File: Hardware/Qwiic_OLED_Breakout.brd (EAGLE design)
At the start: 27.3 x 34.3 mm, 29 parts

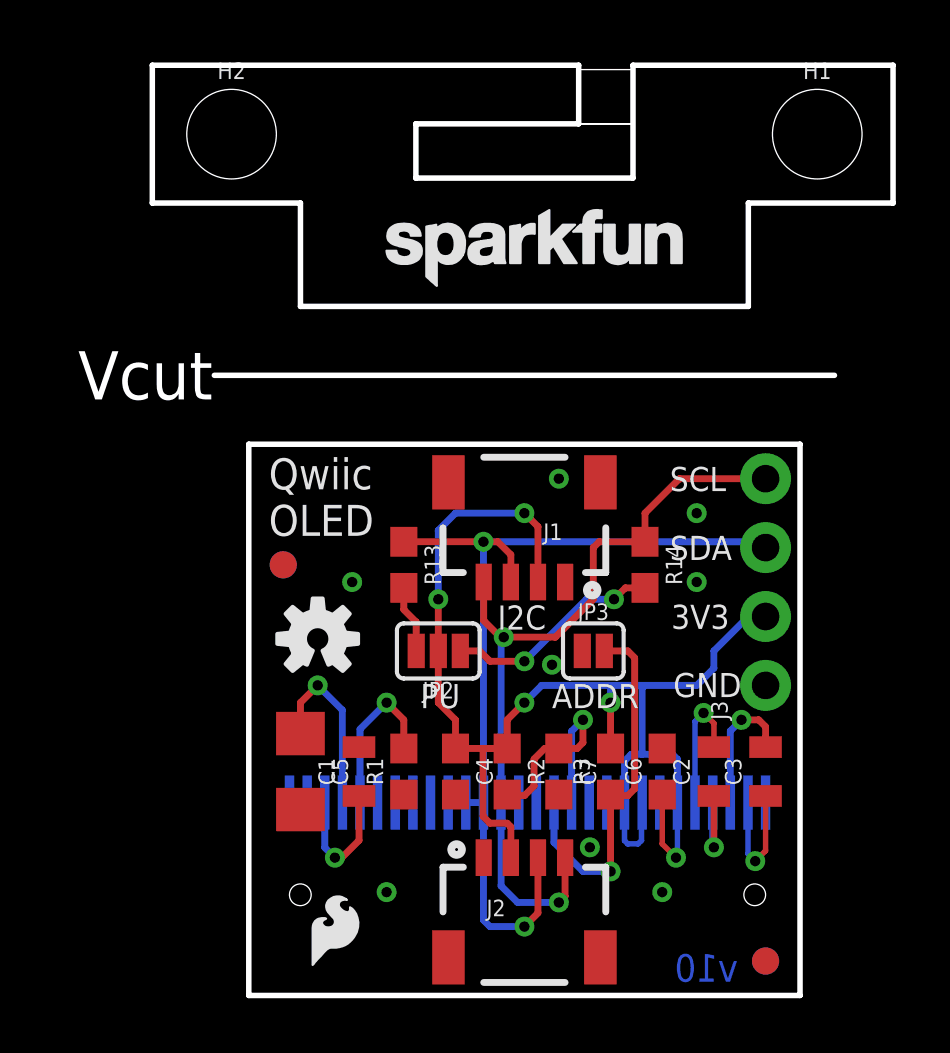
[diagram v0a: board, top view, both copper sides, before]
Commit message: fixed vscore
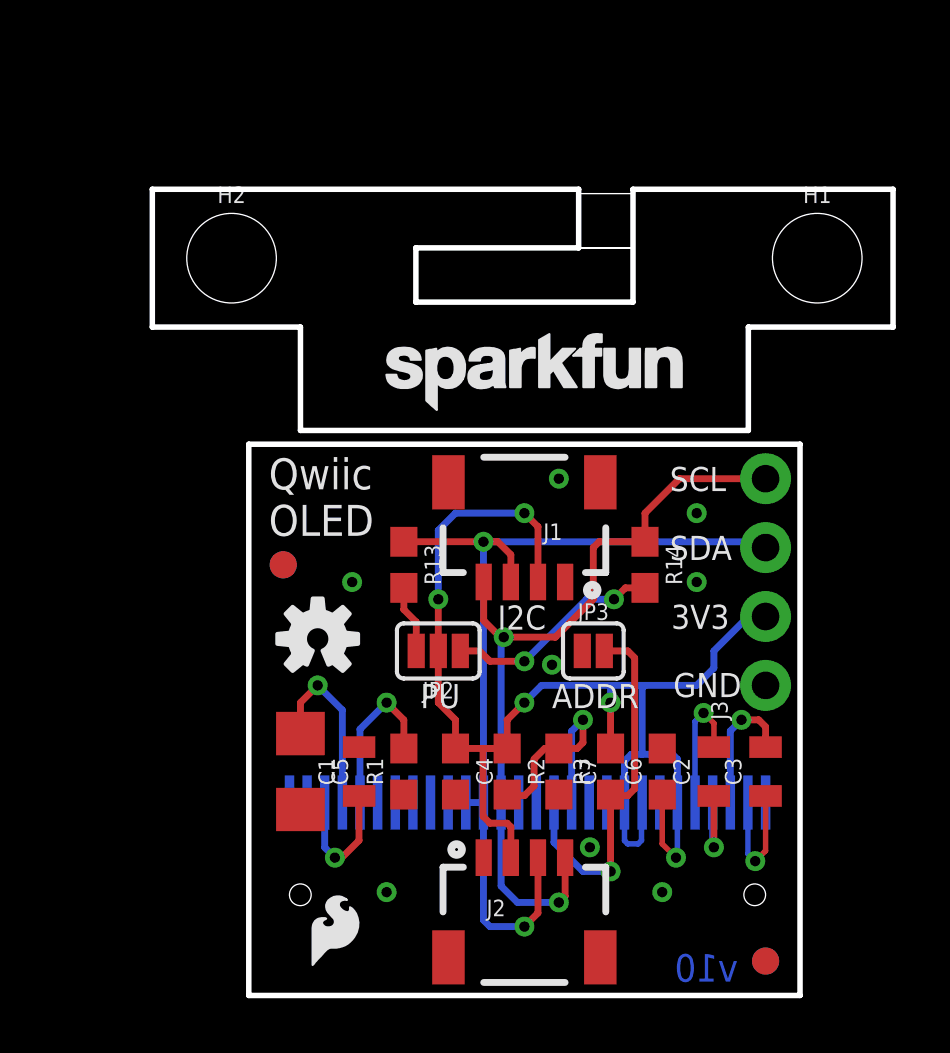
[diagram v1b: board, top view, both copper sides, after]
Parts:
- moved H1 4.57 mm to (21.0, 27.2)
- moved H2 4.57 mm to (-0.64, 27.2)
- moved LOGO4 4.57 mm to (4.57, 21.1)
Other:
- board size 27.3 x 34.3 mm -> 27.3 x 29.7 mm
- board text removed: "Vcut"
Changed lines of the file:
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@@
 <setting verticaltext="up"/>
 </settings>
-<grid distance="0.05" unitdist="inch" unit="inch" style="lines" multiple="1" display="yes" altdistance="0.005" altunitdist="inch" altunit="inch"/>
+<grid distance="0.01" unitdist="inch" unit="inch" style="lines" multiple="1" display="yes" altdistance="0.005" altunitdist="inch" altunit="inch"/>
 <layers>
 <layer number="1" name="Top" color="4" fill="1" visible="yes" active="yes"/>
@@
 <wire x1="0" y1="20.32" x2="0" y2="0" width="0.2032" layer="20"/>
 <wire x1="0" y1="0" x2="20.32" y2="0" width="0.2032" layer="20"/>
-<wire x1="-3.556" y1="34.29" x2="-3.556" y2="29.21" width="0.2032" layer="20"/>
-<wire x1="-3.556" y1="29.21" x2="1.905" y2="29.21" width="0.2032" layer="20"/>
-<wire x1="18.415" y1="29.21" x2="23.749" y2="29.21" width="0.2032" layer="20"/>
-<wire x1="23.749" y1="29.21" x2="23.749" y2="34.29" width="0.2032" layer="20"/>
-<rectangle x1="6.16" y1="30.13" x2="14.16" y2="32.13" layer="46" rot="R180"/>
-<rectangle x1="12.16" y1="32.13" x2="14.16" y2="34.13" layer="46" rot="R180"/>
-<wire x1="12.16" y1="34.29" x2="12.16" y2="32.13" width="0.2032" layer="20"/>
-<wire x1="12.16" y1="32.13" x2="6.16" y2="32.13" width="0.2032" layer="20"/>
-<wire x1="6.16" y1="32.13" x2="6.16" y2="30.13" width="0.2032" layer="20"/>
-<wire x1="6.16" y1="30.13" x2="14.16" y2="30.13" width="0.2032" layer="20"/>
-<wire x1="12.16" y1="34.29" x2="-3.556" y2="34.29" width="0.2032" layer="20"/>
-<wire x1="14.163040625" y1="30.134559375" x2="14.163040625" y2="34.29" width="0.2032" layer="20"/>
-<wire x1="14.163040625" y1="34.29" x2="23.749" y2="34.29" width="0.2032" layer="20"/>
+<wire x1="-3.556" y1="29.718" x2="-3.556" y2="24.638" width="0.2032" layer="20"/>
+<wire x1="-3.556" y1="24.638" x2="1.905" y2="24.638" width="0.2032" layer="20"/>
+<wire x1="18.415" y1="24.638" x2="23.749" y2="24.638" width="0.2032" layer="20"/>
+<wire x1="23.749" y1="24.638" x2="23.749" y2="29.718" width="0.2032" layer="20"/>
+<rectangle x1="6.16" y1="25.558" x2="14.16" y2="27.558" layer="46" rot="R180"/>
+<rectangle x1="12.16" y1="27.558" x2="14.16" y2="29.558" layer="46" rot="R180"/>
+<wire x1="12.16" y1="29.718" x2="12.16" y2="27.558" width="0.2032" layer="20"/>
+<wire x1="12.16" y1="27.558" x2="6.16" y2="27.558" width="0.2032" layer="20"/>
+<wire x1="6.16" y1="27.558" x2="6.16" y2="25.558" width="0.2032" layer="20"/>
+<wire x1="6.16" y1="25.558" x2="14.16" y2="25.558" width="0.2032" layer="20"/>
+<wire x1="12.16" y1="29.718" x2="-3.556" y2="29.718" width="0.2032" layer="20"/>
+<wire x1="14.163040625" y1="25.562559375" x2="14.163040625" y2="29.718" width="0.2032" layer="20"/>
+<wire x1="14.163040625" y1="29.718" x2="23.749" y2="29.718" width="0.2032" layer="20"/>
 <text x="8.89" y="-27.94" size="1.778" layer="51" font="vector">Joel Bartlett</text>
-<dimension x1="-3.81" y1="34.29" x2="-3.81" y2="0" x3="-15.24" y3="17.145" textsize="1.778" layer="47" unit="inch"/>
-<dimension x1="-3.556" y1="34.29" x2="23.749" y2="34.29" x3="10.0965" y3="40.64" textsize="1.778" layer="47" unit="inch"/>
-<dimension x1="-0.635" y1="31.75" x2="20.955" y2="31.75" x3="10.16" y3="36.83" textsize="1.778" layer="47" unit="inch"/>
-<dimension x1="0" y1="0" x2="0" y2="31.75" x3="-11.43" y3="15.875" textsize="1.778" layer="47" unit="inch"/>
+<dimension x1="-3.81" y1="29.718" x2="-3.81" y2="0" x3="-15.24" y3="14.859" textsize="1.778" layer="47" unit="inch"/>
+<dimension x1="-3.556" y1="29.718" x2="23.749" y2="29.718" x3="10.0965" y3="36.068" textsize="1.778" layer="47" unit="inch"/>
+<dimension x1="-0.635" y1="27.178" x2="20.955" y2="27.178" x3="10.16" y3="32.258" textsize="1.778" layer="47" unit="inch"/>
+<dimension x1="0" y1="0" x2="0" y2="27.178" x3="-11.43" y3="13.589" textsize="1.778" layer="47" unit="inch"/>
 <text x="12.7" y="-30.48" size="1.778" layer="51" font="vector">Andy England</text>
-<wire x1="-1.27" y1="22.86" x2="21.59" y2="22.86" width="0.2032" layer="20"/>
-<wire x1="1.905" y1="29.21" x2="1.905" y2="25.4" width="0.2032" layer="20"/>
-<wire x1="1.905" y1="25.4" x2="18.415" y2="25.4" width="0.2032" layer="20"/>
-<wire x1="18.415" y1="25.4" x2="18.415" y2="29.21" width="0.2032" layer="20"/>
+<wire x1="1.905" y1="24.638" x2="1.905" y2="20.828" width="0.2032" layer="20"/>
+<wire x1="1.905" y1="20.828" x2="18.415" y2="20.828" width="0.2032" layer="20"/>
+<wire x1="18.415" y1="20.828" x2="18.415" y2="24.638" width="0.2032" layer="20"/>
 <wire x1="0" y1="20.32" x2="20.32" y2="20.32" width="0.2032" layer="20"/>
-<text x="-3.81" y="22.86" size="1.778" layer="20" align="center">Vcut</text>
-<dimension x1="-6.35" y1="22.86" x2="-6.35" y2="0" x3="-7.62" y3="11.43" textsize="1.778" layer="20" unit="inch"/>
 </plain>
 <attributes>
@@
 </element>
 <element name="JP2" library="SparkFun-Jumpers" package="SMT-JUMPER_3_2-NC_PASTE_SILK" value="" x="6.985" y="12.7" rot="R180"/>
-<element name="H1" library="SparkFun-Hardware" package="STAND-OFF" value="STAND-OFF" x="20.955" y="31.75"/>
-<element name="H2" library="SparkFun-Hardware" package="STAND-OFF" value="STAND-OFF" x="-0.635" y="31.75"/>
+<element name="H1" library="SparkFun-Hardware" package="STAND-OFF" value="STAND-OFF" x="20.955" y="27.178"/>
+<element name="H2" library="SparkFun-Hardware" package="STAND-OFF" value="STAND-OFF" x="-0.635" y="27.178"/>
 <element name="JP3" library="SparkFun-Jumpers" package="SMT-JUMPER_2_NO_SILK" value="" x="12.7" y="12.7"/>
 <element name="LOGO1" library="SparkFun-Aesthetics" package="REVISION" value="REVISION" x="-6.35" y="-30.48"/>
 <element name="LOGO2" library="SparkFun-Aesthetics" package="SFE_LOGO_FLAME_.1" value="SFE_LOGO_FLAME.1_INCH" x="2.032" y="0.762"/>
-<element name="LOGO4" library="SparkFun-Aesthetics" package="SFE_LOGO_NAME_.1" value="SFE_LOGO_NAME.1_INCH" x="4.572" y="25.654"/>
+<element name="LOGO4" library="SparkFun-Aesthetics" package="SFE_LOGO_NAME_.1" value="SFE_LOGO_NAME.1_INCH" x="4.572" y="21.082"/>
 <element name="FID3" library="SparkFun-Aesthetics" package="FIDUCIAL-1X2" value="FIDUCIAL1X2" x="1.27" y="15.875" rot="MR0"/>
 <element name="FID4" library="SparkFun-Aesthetics" package="FIDUCIAL-1X2" value="FIDUCIAL1X2" x="19.05" y="1.27" rot="MR0"/>
